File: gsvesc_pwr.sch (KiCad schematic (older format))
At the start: 45 parts, among them J10 PHASE_C, J11 PHASE_B, J12 NTC, J9 PHASE_A, Q1 TPH2R608NH,L1Q, Q2 TPH2R608NH,L1Q, Q3 TPH2R608NH,L1Q, Q4 TPH2R608NH,L1Q, Q5 TPH2R608NH,L1Q, Q6 TPH2R608NH,L1Q, U4 INA240A2, U5 INA240A2, U6 INA240A2, U7 SN74LVC1G66DBVR, U8 SN74LVC1G66DBVR, U9 SN74LVC1G66DBVR

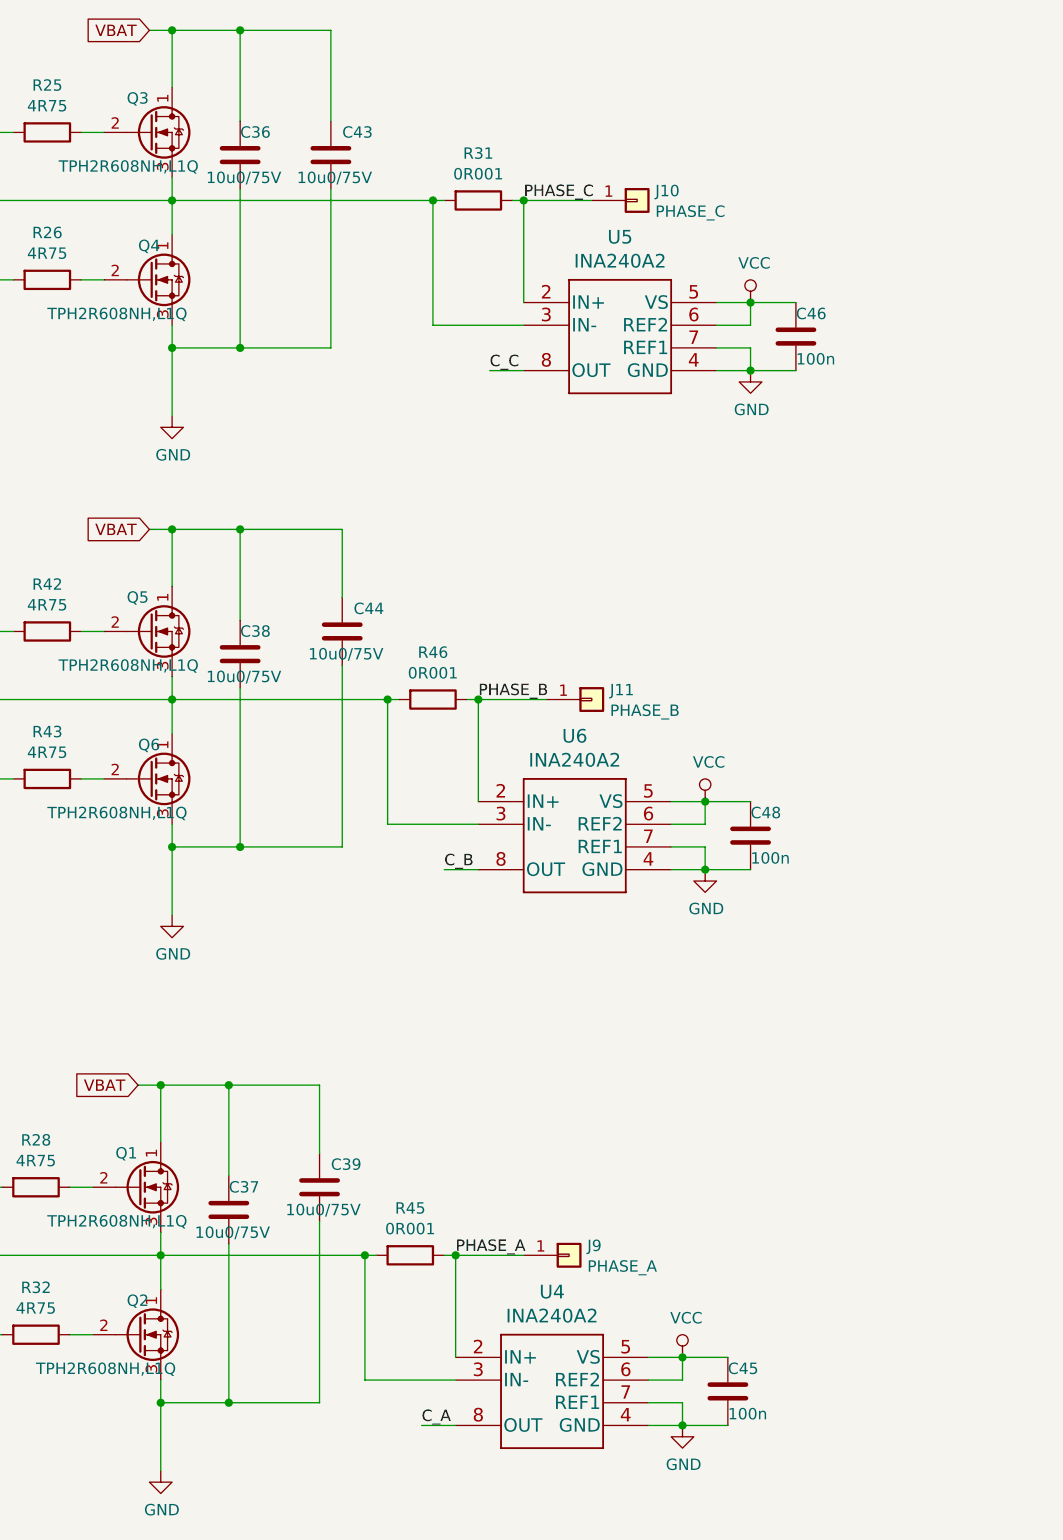
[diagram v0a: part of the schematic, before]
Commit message: temp
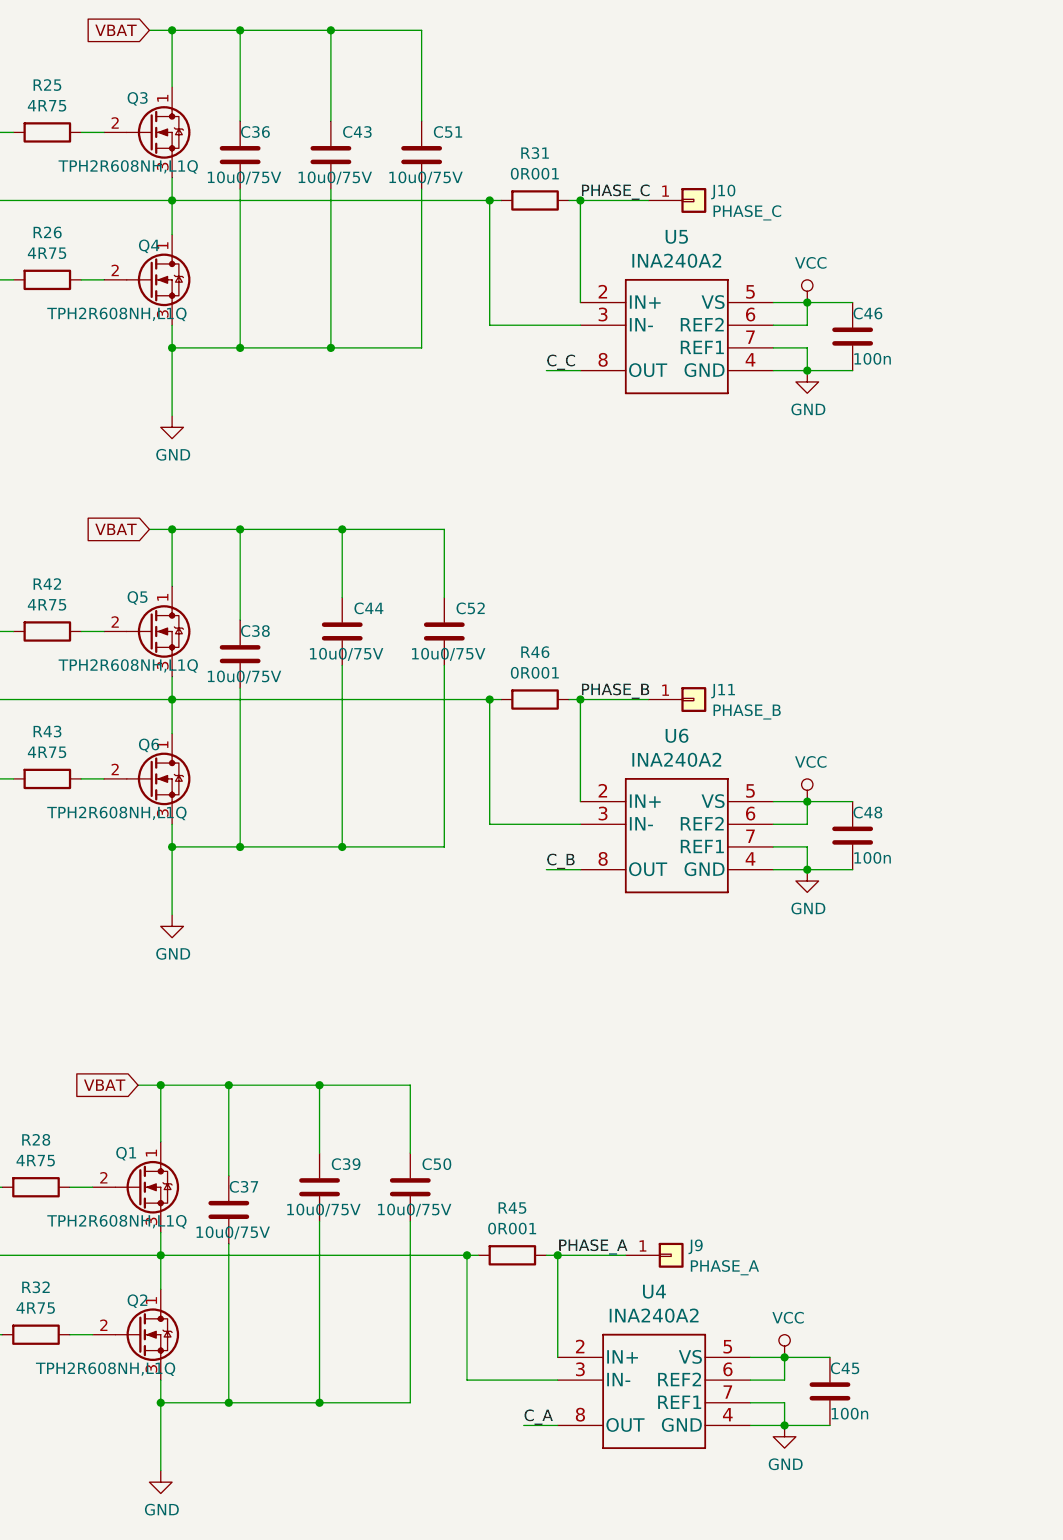
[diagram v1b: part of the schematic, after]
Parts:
- added C50, C51, C52: 10u0/75V, Capacitor_SMD:C_1210_3225Metric, symbol Device:C
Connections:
- net GND: now also C50.2, C51.2, C52.2
- net VBAT: now also C50.1, C51.1, C52.1
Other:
- moved on the sheet: C45, C46, C48, J10, J11, J9, R31, R45, R46, U4, U5, U6
